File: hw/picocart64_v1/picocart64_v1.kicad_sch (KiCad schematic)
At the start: 0 parts

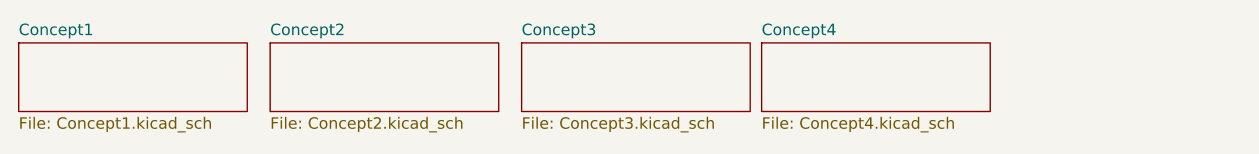
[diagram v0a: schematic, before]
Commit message: hw: Concept5 (is this the one??)
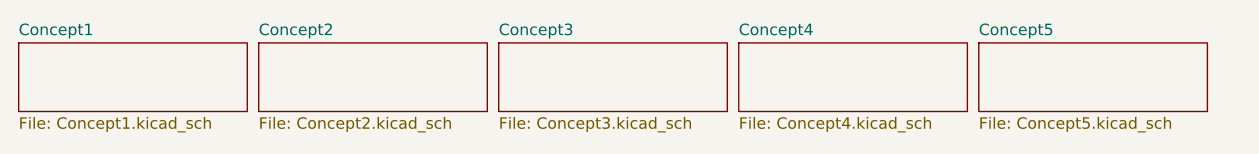
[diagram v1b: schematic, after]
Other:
- added sheet Concept5 (Concept5.kicad_sch)
